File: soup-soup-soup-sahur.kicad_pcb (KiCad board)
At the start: 2 copper layers, 70 x 100 mm, 13 parts, among them J1 USB_C_Receptacle_USB2.0_14P, U1 NT3H2111W0FHKH

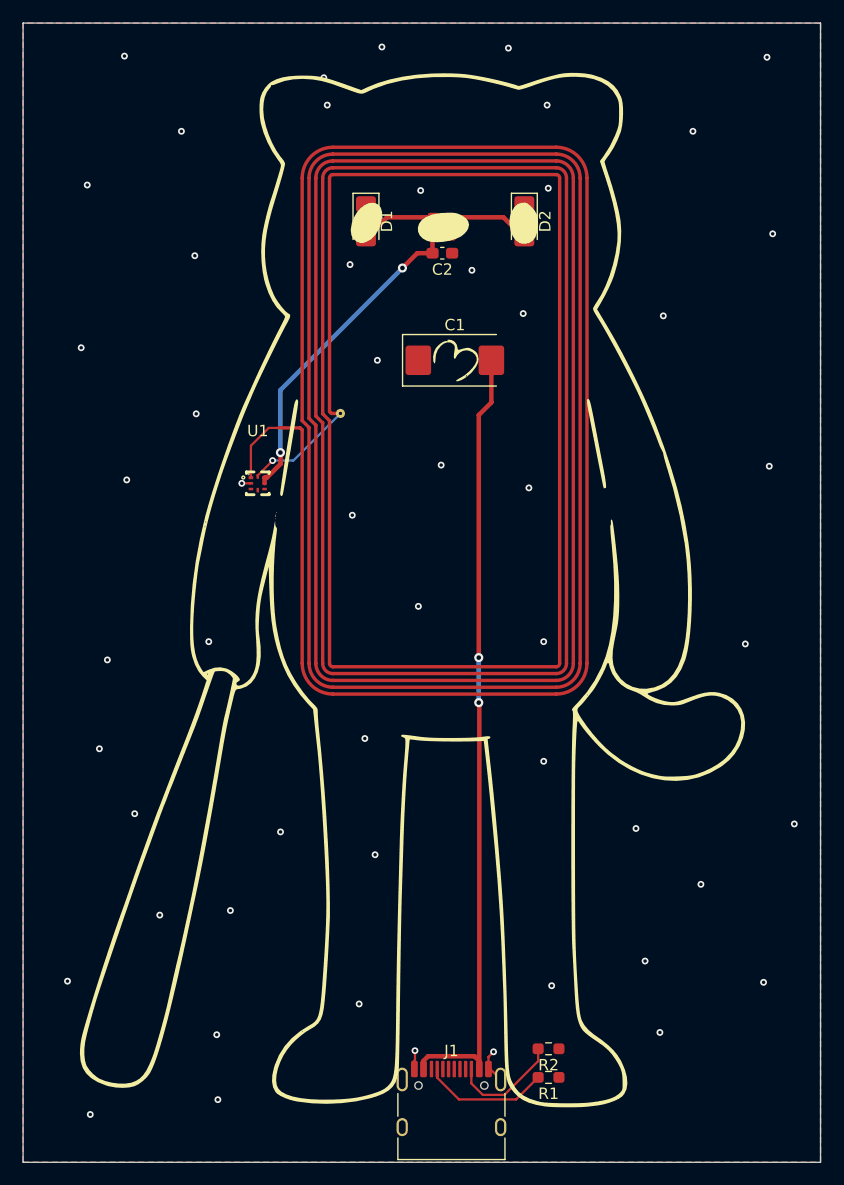
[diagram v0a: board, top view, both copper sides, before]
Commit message: triple s but better
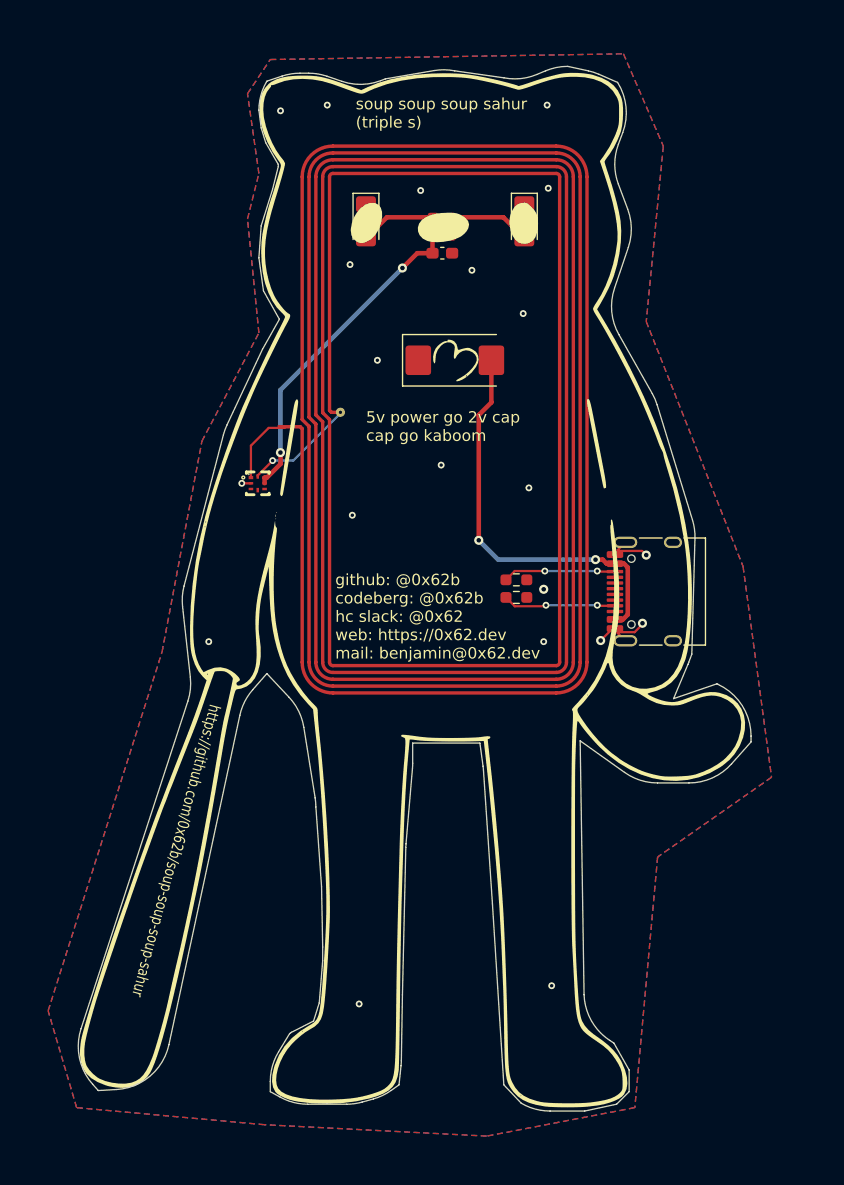
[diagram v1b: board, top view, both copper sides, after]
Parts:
- removed the G*** at (102.9, 81.9)
- moved J1 49.5 mm to (122.8, 85.2), turned to 90 degrees
- moved R1 42.2 mm to (110.1, 85.7)
- moved R2 41.3 mm to (110.1, 84.2)
- moved ANT1 0.10 mm to (103.8, 70.1)
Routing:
- net /explodey thing: track 69.4 -> 35.8 mm
- net GND: track 5.73 -> 11.3 mm, vias 54 -> 21
- net Net-(J1-CC1): track 11.2 -> 9.95 mm, vias 0 -> 2
- net Net-(J1-CC2): track 9.85 -> 9.91 mm, vias 0 -> 2
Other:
- board size 70 x 100 mm -> 59.1 x 91.7 mm
- board text added: "5v power go 2v cap cap go kaboom"
- board text added: "github: @0x62b codeberg: @0x62b hc slack: @0x62 web: https://0x62.dev mail: benjamin@0x62.dev"
- board text added: "soup soup soup sahur (triple s)"
- board text removed: "github: @0x62b codeberg: @0x62b hc slack: @0x62 signal: benjamin.492 web: https://0x62.dev mail: benjamin@0x62.dev"
